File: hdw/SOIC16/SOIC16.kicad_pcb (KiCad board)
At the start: 2 copper layers, 20.3 x 12.7 mm, 3 parts, among them J16 SOIC16-P01-P08, J17 SOIC16-P09-P16, U5 CH340C

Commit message: Save changes at: 1748167978
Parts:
- J16, J17: moved to B.Cu
- turned J16 to -90 degrees
- turned J17 to 90 degrees

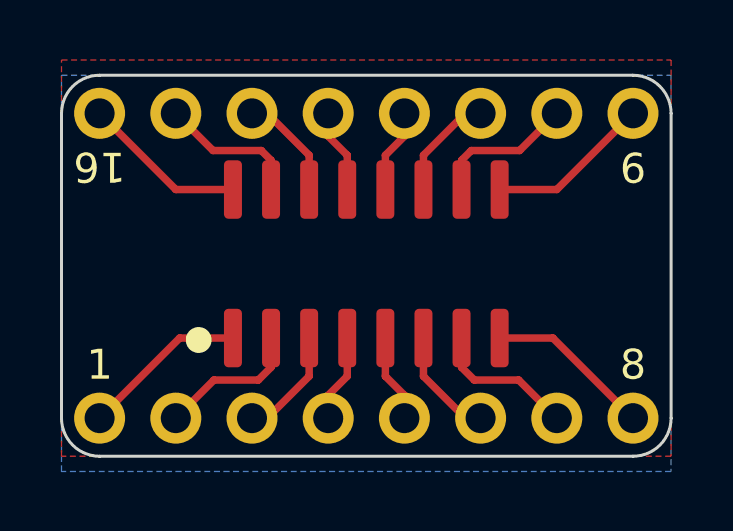
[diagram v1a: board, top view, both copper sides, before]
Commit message: Save changes at: 1748380927
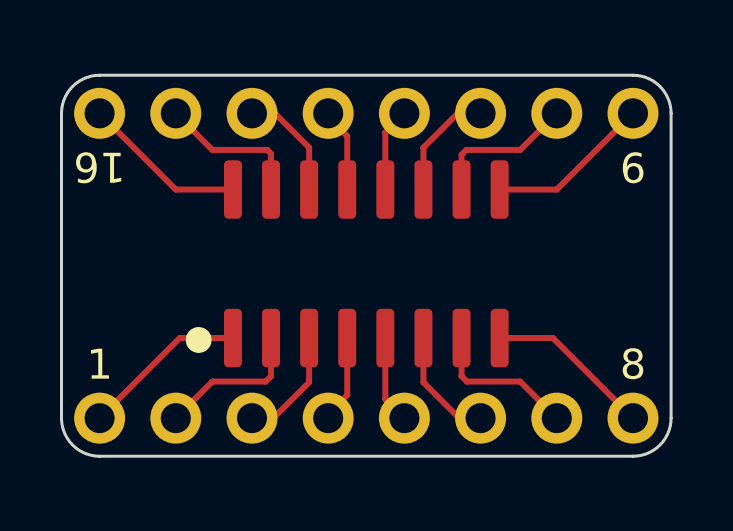
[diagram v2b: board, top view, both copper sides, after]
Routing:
- removed copper zone on B.Cu, net (none)
- removed copper zone on F.Cu, net (none)
